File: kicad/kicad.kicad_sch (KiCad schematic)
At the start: 0 parts

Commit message: Session #1: README update, designed the whole board lol
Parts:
- added BT2: Battery_Cell, Battery:BatteryHolder_MYOUNG_BS-07-A1BJ001_CR2032, symbol Device:Battery_Cell
- added D1, D10, D2, D3, D4, D5, D6, D7, D8, D9: LED, LED_THT:LED_D5.0mm, symbol Device:LED
- added R1: 220, Resistor_THT:R_Axial_DIN0207_L6.3mm_D2.5mm_P10.16mm_Horizontal, symbol Device:R
- added R2: 10k, Resistor_THT:R_Axial_DIN0207_L6.3mm_D2.5mm_P10.16mm_Horizontal, symbol Device:R
- added RV1: Trimpot, Potentiometer_THT:Potentiometer_Runtron_RM-065_Vertical, symbol Device:R_Potentiometer_Trim
- added SW1: SW_Push, Button_Switch_THT:SW_PUSH_6mm, symbol Switch:SW_Push
- added U2: ATtiny85-20P, Package_DIP:DIP-8_W7.62mm, symbol MCU_Microchip_ATtiny:ATtiny85-20P
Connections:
- new net: D1.2 (A), D10.2 (A), D2.2 (A), D3.2 (A), D4.2 (A), D5.2 (A), D6.2 (A), D7.2 (A), D8.2 (A), D9.2 (A), R1.2
- new net: R2.2, RV1.2, U2.2 (XTAL1/PB3)
- new net: BT2.1 (+), R2.1, U2.8 (VCC)
- new net: R1.1, U2.6 (PB1)
- new net: SW1.2, U2.7 (PB2)
- new net GND: BT2.2 (-), D1.1 (K), D10.1 (K), D2.1 (K), D3.1 (K), D4.1 (K), D5.1 (K), D6.1 (K), D7.1 (K), D8.1 (K), D9.1 (K), RV1.1, RV1.3, SW1.1, U2.4 (GND)
- no-connect marks 0 -> 3

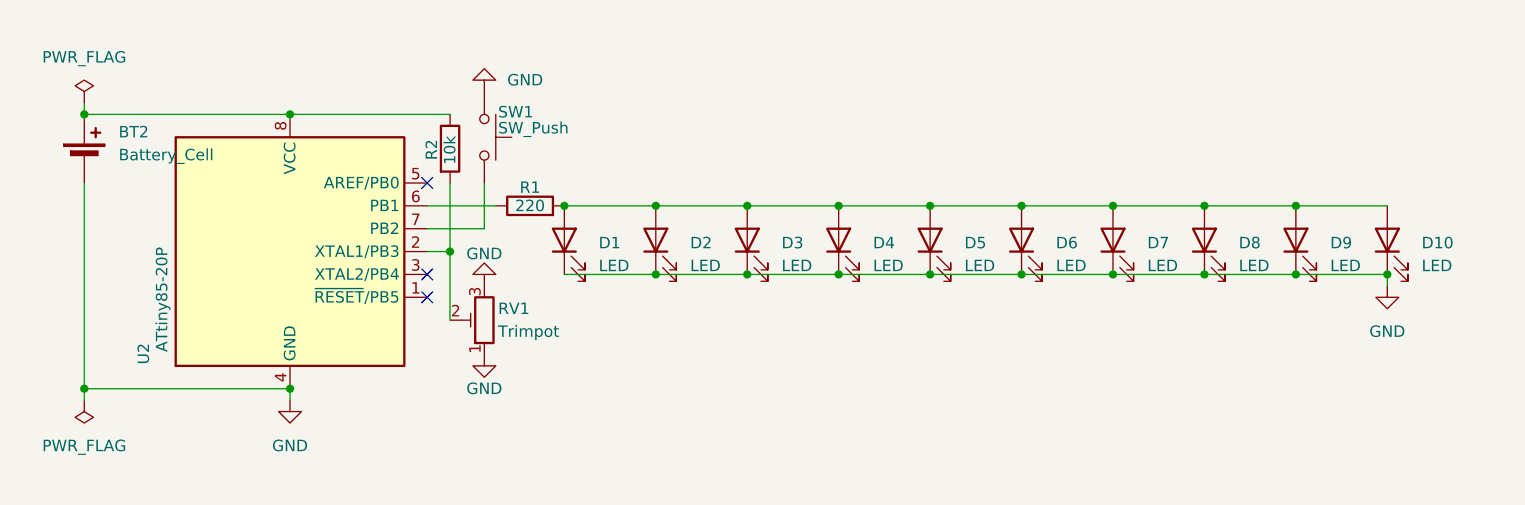
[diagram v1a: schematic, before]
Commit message: Session #4: Trimpot brightness control, README update
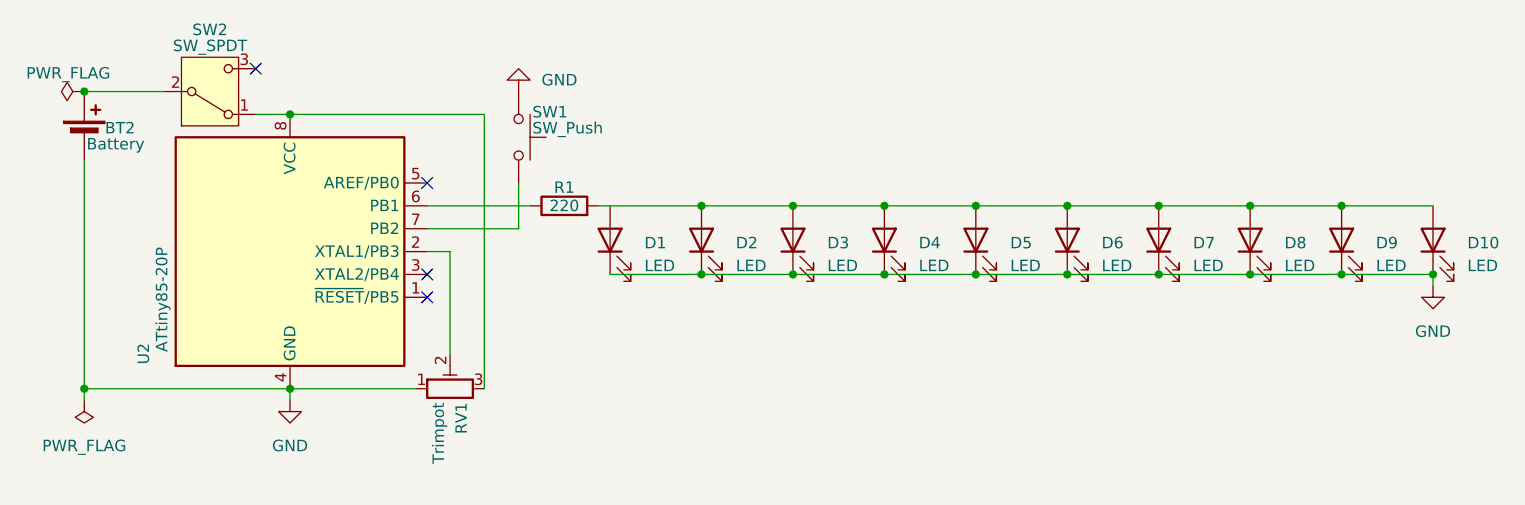
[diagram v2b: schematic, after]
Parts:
- removed R2: 10k, Resistor_THT:R_Axial_DIN0207_L6.3mm_D2.5mm_P10.16mm_Horizontal, symbol Device:R
- added SW2: SW_SPDT, Button_Switch_THT:SW_Slide-03_Wuerth-WS-SLTV_10x2.5x6.4_P2.54mm, symbol Switch:SW_SPDT
- BT2: value Battery_Cell -> Battery
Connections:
- net GND: no longer RV1.3
- net at U2.8 (VCC): now also RV1.3, SW2.1 (A); no longer BT2.1 (+)
- new net: BT2.1 (+), SW2.2 (B)
- no-connect marks 3 -> 4
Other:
- moved on the sheet: BT2, D1, D10, D2, D3, D4, D5, D6, D7, D8, D9, R1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
